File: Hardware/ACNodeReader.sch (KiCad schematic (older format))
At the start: 34 parts, among them J1 Conn_01x08_Male, J2 AVR-ISP-6, J3 Conn_01x04_Female, J4 Conn_01x02_Male, J5 Conn_01x04_Female, J6 Conn_01x04_Male, J7 Conn_01x04_Male, U1 L78L05_SOT89, U2 ATmega88PB-AU, U3 ISL8489EIBZ, U4 LM75C, Y1 Crystal_GND24

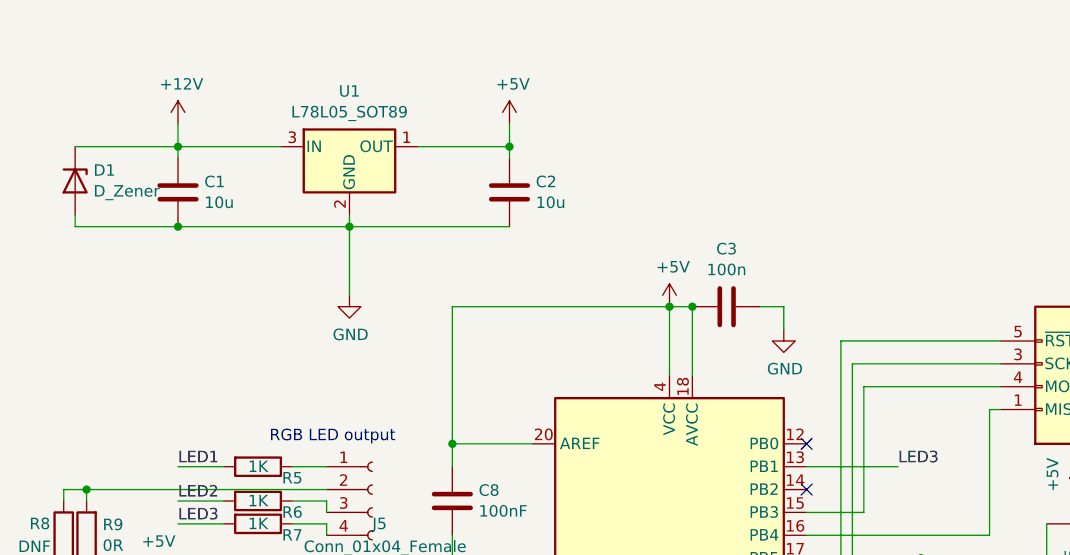
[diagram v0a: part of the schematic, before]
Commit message: Added some notes to schematic and updated firmware with new board support
getting there!
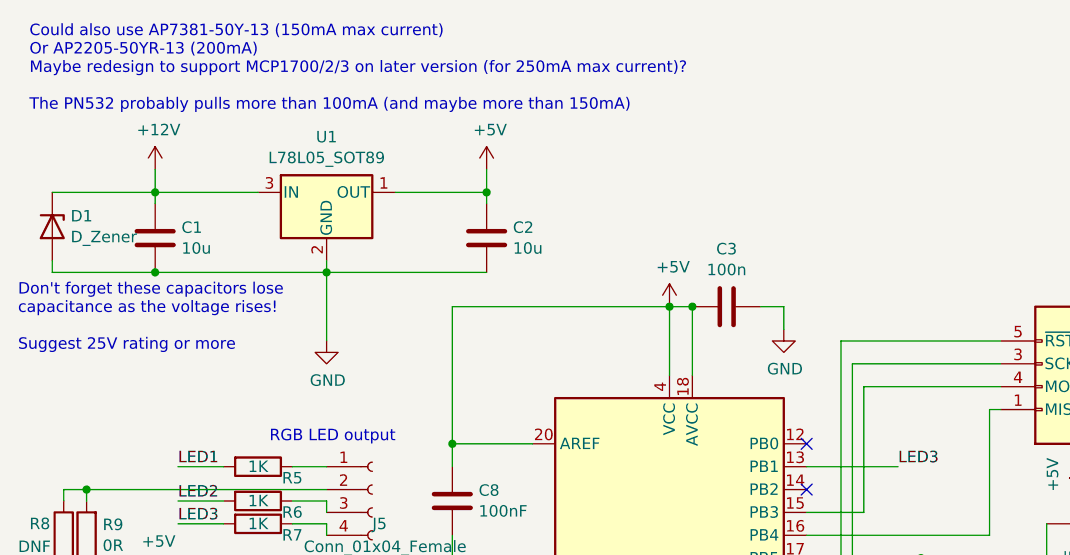
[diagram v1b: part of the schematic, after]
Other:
- note added: "Could also use AP7381-50Y-13 (150mA max current)\nOr AP2205-50YR-13 (200mA)\nMaybe redesign to support MCP1700/2/3 on later version (for 250mA max current)?\n\nThe PN532 probably pulls more than 100mA (and maybe more than 150mA)\n"
- note added: "Don't forget these capacitors lose\ncapacitance as the voltage rises!\n\nSuggest 25V rating or more\n"
- moved on the sheet: C1, C2, D1, U1
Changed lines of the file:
@@
 L Regulator_Linear:L78L05_SOT89 U1
 U 1 1 5D3D7904
-P 2050 1150
-F 0 "U1" H 2050 1392 50  0000 C CNN
-F 1 "L78L05_SOT89" H 2050 1301 50  0000 C CNN
-F 2 "Package_TO_SOT_SMD:SOT-89-3" H 2050 1350 50  0001 C CIN
-F 3 "http://www.st.com/content/ccc/resource/technical/document/datasheet/15/55/e5/aa/23/5b/43/fd/CD00000446.pdf/files/CD00000446.pdf/jcr:content/translations/en.CD00000446.pdf" H 2050 1100 50  0001 C CNN
-	1    2050 1150
+P 1950 1350
+F 0 "U1" H 1950 1592 50  0000 C CNN
+F 1 "L78L05_SOT89" H 1950 1501 50  0000 C CNN
+F 2 "Package_TO_SOT_SMD:SOT-89-3" H 1950 1550 50  0001 C CIN
+F 3 "http://www.st.com/content/ccc/resource/technical/document/datasheet/15/55/e5/aa/23/5b/43/fd/CD00000446.pdf/files/CD00000446.pdf/jcr:content/translations/en.CD00000446.pdf" H 1950 1300 50  0001 C CNN
+	1    1950 1350
 	1    0    0    -1
 $EndComp
@@
 L power:GND #PWR0103
 U 1 1 5D3D8510
-P 2050 1800
-F 0 "#PWR0103" H 2050 1550 50  0001 C CNN
-F 1 "GND" H 2055 1627 50  0000 C CNN
-F 2 "" H 2050 1800 50  0001 C CNN
-F 3 "" H 2050 1800 50  0001 C CNN
-	1    2050 1800
+P 1950 2000
+F 0 "#PWR0103" H 1950 1750 50  0001 C CNN
+F 1 "GND" H 1955 1827 50  0000 C CNN
+F 2 "" H 1950 2000 50  0001 C CNN
+F 3 "" H 1950 2000 50  0001 C CNN
+	1    1950 2000
 	1    0    0    -1
 $EndComp
@@
 L power:+12V #PWR0104
 U 1 1 5D3D8CA0
-P 1300 1050
-F 0 "#PWR0104" H 1300 900 50  0001 C CNN
-F 1 "+12V" H 1315 1223 50  0000 C CNN
-F 2 "" H 1300 1050 50  0001 C CNN
-F 3 "" H 1300 1050 50  0001 C CNN
-	1    1300 1050
+P 1200 1250
+F 0 "#PWR0104" H 1200 1100 50  0001 C CNN
+F 1 "+12V" H 1215 1423 50  0000 C CNN
+F 2 "" H 1200 1250 50  0001 C CNN
+F 3 "" H 1200 1250 50  0001 C CNN
+	1    1200 1250
 	1    0    0    -1
 $EndComp
@@
 L power:+5V #PWR0105
 U 1 1 5D3D9614
-P 2750 1050
-F 0 "#PWR0105" H 2750 900 50  0001 C CNN
-F 1 "+5V" H 2765 1223 50  0000 C CNN
-F 2 "" H 2750 1050 50  0001 C CNN
-F 3 "" H 2750 1050 50  0001 C CNN
-	1    2750 1050
-	1    0    0    -1
-$EndComp
-Wire Wire Line
-	1300 1050 1300 1150
-Wire Wire Line
-	2750 1150 2750 1050
-Wire Wire Line
-	2050 1800 2050 1500
-Wire Wire Line
-	2750 1200 2750 1150
-Connection ~ 2750 1150
-Wire Wire Line
-	2750 1500 2050 1500
-Connection ~ 2050 1500
-Wire Wire Line
-	2050 1500 2050 1450
-Wire Wire Line
-	1300 1200 1300 1150
-Connection ~ 1300 1150
+P 2650 1250
+F 0 "#PWR0105" H 2650 1100 50  0001 C CNN
+F 1 "+5V" H 2665 1423 50  0000 C CNN
+F 2 "" H 2650 1250 50  0001 C CNN
+F 3 "" H 2650 1250 50  0001 C CNN
+	1    2650 1250
+	1    0    0    -1
+$EndComp
+Wire Wire Line
+	1200 1250 1200 1350
+Wire Wire Line
+	2650 1350 2650 1250
+Wire Wire Line
+	1950 2000 1950 1700
+Wire Wire Line
+	2650 1400 2650 1350
+Connection ~ 2650 1350
+Connection ~ 1950 1700
+Wire Wire Line
+	1950 1700 1950 1650
+Wire Wire Line
+	1200 1400 1200 1350
+Connection ~ 1200 1350
 Wire Wire Line
 	4050 4250 4600 4250
@@
 i2c_SDA
 Wire Wire Line
-	1300 1150 1750 1150
-Wire Wire Line
-	1300 1500 2050 1500
-Wire Wire Line
-	2350 1150 2750 1150
+	1200 1350 1650 1350
+Wire Wire Line
+	1200 1700 1950 1700
+Wire Wire Line
+	2250 1350 2650 1350
 $Comp
 L ACNodeReader-rescue:ATmega88PB-AU-MCU_Microchip_ATmega U2
@@
 L Device:C C1
 U 1 1 5EE74DE3
-P 1300 1350
-F 0 "C1" H 1415 1396 50  0000 L CNN
-F 1 "10u" H 1415 1305 50  0000 L CNN
-F 2 "Capacitor_SMD:C_0805_2012Metric" H 1338 1200 50  0001 C CNN
-F 3 "~" H 1300 1350 50  0001 C CNN
-	1    1300 1350
+P 1200 1550
+F 0 "C1" H 1315 1596 50  0000 L CNN
+F 1 "10u" H 1315 1505 50  0000 L CNN
+F 2 "Capacitor_SMD:C_0805_2012Metric" H 1238 1400 50  0001 C CNN
+F 3 "~" H 1200 1550 50  0001 C CNN
+	1    1200 1550
 	1    0    0    -1
 $EndComp
@@
 L Device:C C2
 U 1 1 5EE7545C
-P 2750 1350
-F 0 "C2" H 2865 1396 50  0000 L CNN
-F 1 "10u" H 2865 1305 50  0000 L CNN
-F 2 "Capacitor_SMD:C_0805_2012Metric" H 2788 1200 50  0001 C CNN
-F 3 "~" H 2750 1350 50  0001 C CNN
-	1    2750 1350
+P 2650 1550
+F 0 "C2" H 2765 1596 50  0000 L CNN
+F 1 "10u" H 2765 1505 50  0000 L CNN
+F 2 "Capacitor_SMD:C_0805_2012Metric" H 2688 1400 50  0001 C CNN
+F 3 "~" H 2650 1550 50  0001 C CNN
+	1    2650 1550
 	1    0    0    -1
 $EndComp
@@
 L Device:D_Zener D1
 U 1 1 5F745A0A
-P 850 1300
-F 0 "D1" V 804 1380 50  0000 L CNN
-F 1 "D_Zener" V 895 1380 50  0000 L CNN
-F 2 "Diode_SMD:D_SOD-323F" H 850 1300 50  0001 C CNN
-F 3 "~" H 850 1300 50  0001 C CNN
-	1    850  1300
-	0    1    1    0
-$EndComp
-Wire Wire Line
-	1300 1150 850  1150
-Wire Wire Line
-	1300 1500 850  1500
-Wire Wire Line
-	850  1500 850  1450
-Connection ~ 1300 1500
+P 750 1500
+F 0 "D1" V 704 1580 50  0000 L CNN
+F 1 "D_Zener" V 795 1580 50  0000 L CNN
+F 2 "Diode_SMD:D_SOD-323F" H 750 1500 50  0001 C CNN
+F 3 "~" H 750 1500 50  0001 C CNN
+	1    750  1500
+	0    1    1    0
+$EndComp
+Wire Wire Line
+	1200 1350 750  1350
+Wire Wire Line
+	1200 1700 750  1700
+Wire Wire Line
+	750  1700 750  1650
+Connection ~ 1200 1700
 Wire Wire Line
 	4600 4700 6100 4700
@@
 NoConn ~ 4050 2450
 NoConn ~ 4050 2650
+Text Notes 650  1000 0    50   ~ 0
+Could also use AP7381-50Y-13 (150mA max current)\nOr AP2205-50YR-13 (200mA)\nMaybe redesign to support MCP1700/2/3 on later version (for 250mA max current)?\n\nThe PN532 probably pulls more than 100mA (and maybe more than 150mA)\n
+Wire Wire Line
+	1950 1700 2650 1700
+Text Notes 600  2050 0    50   ~ 0
+Don't forget these capacitors lose\ncapacitance as the voltage rises!\n\nSuggest 25V rating or more\n
 $EndSCHEMATC
